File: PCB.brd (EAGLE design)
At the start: 127 x 44.5 mm, 45 parts, among them IC1 PIC16F1826/27SO, IC2 MAX3467CPA, U1 +12v, Y1 ASL-16.000MHZ-L-C-S-50-T

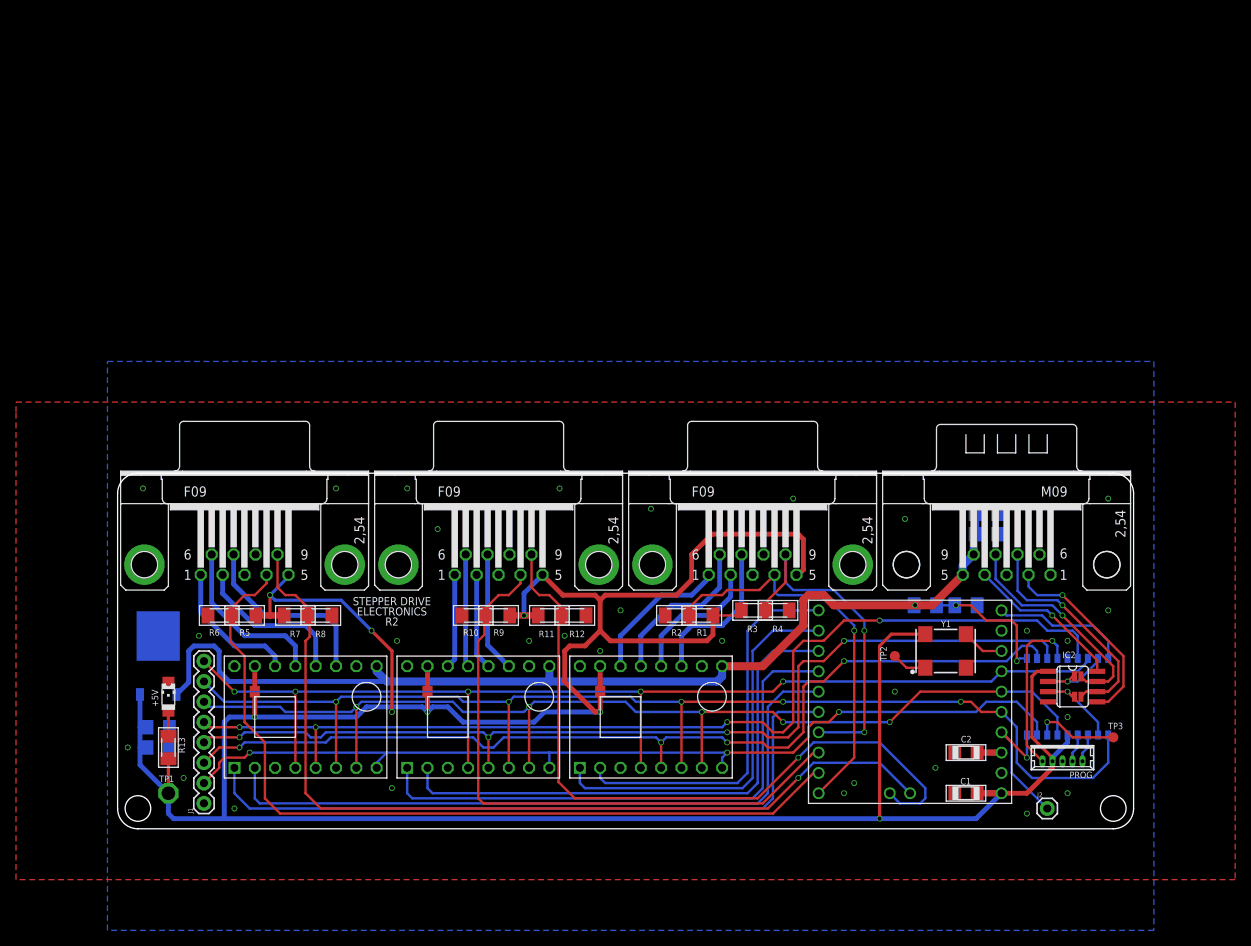
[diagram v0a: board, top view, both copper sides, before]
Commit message: Updating PCB design
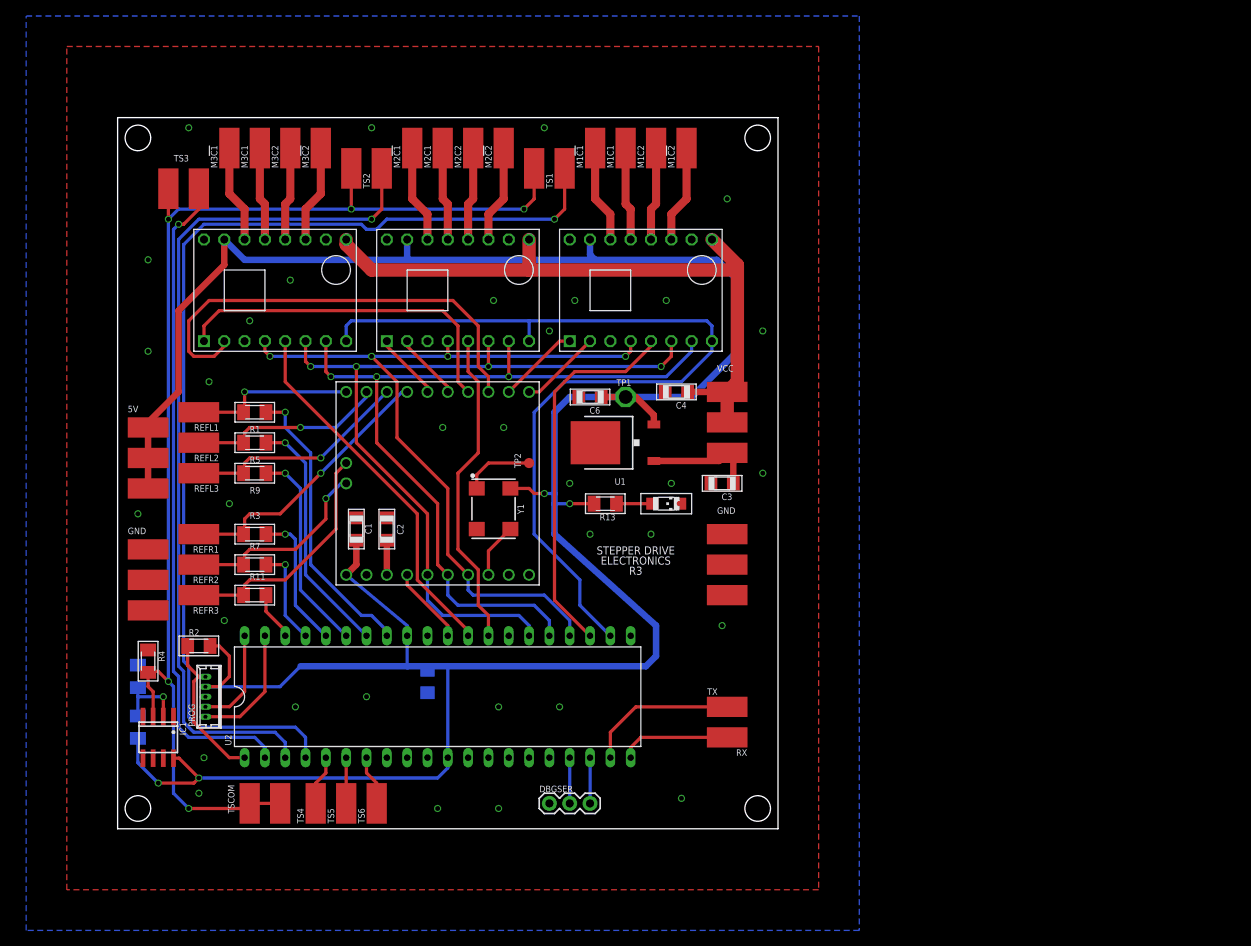
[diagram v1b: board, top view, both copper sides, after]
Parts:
- removed IC2: MAX3467CPA, maxim:SO08
- removed J1: (no value), SparkFun-Connectors:1X08
- removed J2: (no value), SparkFun-Connectors:1X01
- removed JP1, JP2, JP3, JP4, JP5: JUMPER-SMT_2_NO_NO-SILK, SparkFun-Jumpers:SMT-JUMPER_2_NO_NO-SILK
- removed R10, R12, R14, R15: (no value), resistor:M1206
- removed TP3: PTR1B1,27, testpad:B1,27
- removed X1, X2, X3: (no value), con-subd:F09HP
- removed X4: (no value), con-subd:M09H
- added 5V@1, 5V@2, 5V@3, GND@1, GND@2, GND@3, GND@4, GND@5, GND@6, M1!C1, M1!C2, M1C1, M1C2, M2!C1, M2!C2, M2C1, M2C2, M3!C1, M3!C2, M3C1, M3C2, REFL1, REFL2, REFL3, REFR1, REFR2, REFR3, RX, TS1, TS2, TS3, TS4, TS5, TS6, TSCOM@1, TSCOM@2, TSCOM@3, TSCOM@4, TSCOM@5, TX, VCC@1, VCC@2, VCC@3: WIREPADSMD2,54-5,08, wirepad:SMD2,54-5,08
- added DBGSER: (no value), SparkFun-Connectors:1X03
- added U2: PIC18F47Q84, FRC696:DIL40
- C3, C5: value (none) -> 0.1uF
- C4, C6: value (none) -> 1uF
- IC1: value PIC16F1826/27SO -> LM393D; device microchip:SO-18W -> linear:SO08
- PROG: value 53047-05 -> PIC-PROG047; device con-molex:53047-05 -> FRC696:53047-05
- R1, R11, R2, R3, R5, R7, R9: value (none) -> 5k
- R13: value (none) -> 330
- R4, R6: value (none) -> 10k
- R8: value (none) -> 2.2k
- moved IC1 113.8 mm to (5.08, 11.4), flipped to the top
- moved PROG 107.0 mm to (11.4, 16.5), turned to 90 degrees
- moved C1 83.0 mm to (29.8, 37.5), turned to 90 degrees
- moved R4 79.0 mm to (3.81, 21.0), turned to 270 degrees
- moved C2 77.6 mm to (33.7, 37.5), turned to 270 degrees
- moved TP1 75.6 mm to (63.5, 54.0)
- moved C6 69.5 mm to (59.1, 54.0), flipped to the top
- moved U$1 66.8 mm to (38.7, 43.2), turned to 90 degrees
- moved LED1 66.7 mm to (68.6, 40.6), turned to 270 degrees
- moved U1 63.1 mm to (62.2, 48.3), flipped to the top, turned to 90 degrees
- moved R3 63.0 mm to (17.1, 36.8), turned to 0 degrees
- moved R13 62.5 mm to (61.0, 40.6), turned to 180 degrees
- moved R1 61.4 mm to (17.1, 52.1)
- moved R2 59.8 mm to (10.2, 22.9)
- moved Y1 59.2 mm to (47.0, 40.0), turned to 270 degrees
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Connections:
- removed net N$25: IC1.16, TP3.TP
- removed net N$29: DRV2.P$15, JP4.1
- removed net N$30: DRV1.P$15, JP3.1
- removed net N$31: DRV3.P$15, JP5.1
- removed net N$33: IC1.1, R14.1, R15.2
- removed net RXN: IC2.7, JP2.1, X4.8
- removed net RXP: IC2.8, X4.4
- removed net TXN: IC2.6, JP1.1, X4.7
- removed net TXP: IC2.5, X4.2
- new net DBGRX: DBGSER.3, U2.18
- new net DBGTX: DBGSER.2, U2.17
- new net N$26: IC1.2, R6.1, R8.2
- new net REFL1P: R1.2, U2.33
- new net REFL2P: R5.2, U2.34
- new net REFL3P: R9.2, U2.35
- new net REFR1P: R3.2, U2.36
- new net REFR2P: R7.2, U2.37
- new net REFR3P: R11.2, U2.38
- new net TS1: TS1.1, U2.4
- new net TS2: TS2.1, U2.3
- new net TS3: TS3.1, U2.2
- new net TS4: TS4.1, U2.5
- new net TS5: TS5.1, U2.6
- new net TS6: TS6.1, U2.7
- new net TSCOM: IC1.3, R4.2, TSCOM@1.1, TSCOM@2.1, TSCOM@3.1, TSCOM@4.1, TSCOM@5.1
- new net TSOUT: IC1.1
- net +5V: now also 5V@1.1, 5V@2.1, 5V@3.1, DRV1.P$15, DRV2.P$15, DRV3.P$15, IC1.8, R2.2, R6.2, U2.11, U2.32; no longer IC1.14, IC2.1, JP3.2, JP4.2, JP5.2, R1.2, R11.2, R3.2, R5.2, R7.2, R9.2, X1.5, X2.5, X3.5
- net D1CS: now also U2.23; no longer IC1.2, J1.3
- net D2CS: now also U2.28; no longer IC1.6, J1.5
- net D3CS: now also U2.29; no longer IC1.3, J1.4
- net DRVEN: now also U2.22; no longer IC1.17, J1.2
- net GND: now also DBGSER.1, GND@1.1, GND@2.1, GND@3.1, GND@4.1, GND@5.1, GND@6.1, IC1.4, IC1.6, U2.12, U2.31; no longer IC2.4, J1.1, R10.1, R12.1, R15.1, R2.1, R6.1, X1.8, X2.8, X3.8, X4.1, X4.6
- net MCCS: now also U2.30; no longer IC1.18, J2.1
- net MCINT: no longer IC1.9
- net MISO: now also U2.24; no longer IC1.7, J1.8
- net MOSI: now also U2.25; no longer IC1.15, J1.6
- net N$10: now also M1!C1.1; no longer X1.1
- net N$11: now also M1!C2.1; no longer X1.7
- net N$12: now also M2!C1.1; no longer X2.1
- net N$13: now also M2C2.1; no longer X2.2
- net N$14: now also M2!C2.1; no longer X2.7
- net N$15: now also M2C1.1; no longer X2.6
- net N$16: now also M3!C1.1; no longer X3.1
- net N$17: now also M3C2.1; no longer X3.2
- net N$18: now also M3C1.1; no longer X3.6
- net N$19: now also M3!C2.1; no longer X3.7
- net N$20: now also PROG.4, U2.40; no longer IC1.4, PROG.1
- net N$21: now also PROG.1, R2.1, U2.1; no longer IC1.13, PROG.4
- net N$22: now also U2.39; no longer IC1.12
- net N$8: now also M1C1.1; no longer X1.6
- net N$9: now also M1C2.1; no longer X1.2
- net REFL1: now also REFL1.1; no longer R2.2, X1.4
- net REFL2: now also REFL2.1; no longer R6.2, X2.4
- net REFL3: now also REFL3.1; no longer R10.2, X3.4
- net REFR1: now also REFR1.1; no longer R4.2, X1.9
- net REFR2: now also REFR2.1; no longer R8.2, X2.9
- net REFR3: now also REFR3.1; no longer R12.2, X3.9
- net SCK: now also U2.26; no longer IC1.10, J1.7
- net UARTRX: now also RX.1, U2.20; no longer IC1.8, IC2.2, JP2.2
- net UARTTX: now also TX.1, U2.19; no longer IC1.11, IC2.3, JP1.2
- net VCC: now also VCC@1.1, VCC@2.1, VCC@3.1; no longer R14.2, X4.5, X4.9
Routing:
- net TSCOM: track 0.00 -> 154.8 mm, vias 0 -> 5
- net TS1: track 0.00 -> 132.6 mm, vias 0 -> 1
- net TS2: track 0.00 -> 108.3 mm, vias 0 -> 1
- net D2CS: track 130.0 -> 40.0 mm, vias 4 -> 0
- net REFR2: track 113.0 -> 24.8 mm
- net TS3: track 0.00 -> 82.4 mm, vias 0 -> 1
- net REFL2: track 104.7 -> 24.6 mm, vias 0 -> 1
- net N$4: track 87.9 -> 8.45 mm
- net N$3: track 86.7 -> 8.45 mm
- net D3CS: track 122.3 -> 46.3 mm, vias 4 -> 0
- net D1CS: track 120.5 -> 47.4 mm, vias 4 -> 0
- net REFR3: track 89.8 -> 30.0 mm, vias 1 -> 0
- net REFL3: track 76.5 -> 28.4 mm, vias 0 -> 1
- net SCK: track 150.7 -> 104.2 mm, vias 5 -> 4
- net MISO: track 142.6 -> 101.1 mm, vias 5 -> 4
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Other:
- board size 127 x 44.5 mm -> 82.5 x 88.9 mm
- board text added: "5V"
- board text added: "GND"
- board text added: "R3"
- board text added: "TSCOM"
- board text added: "VCC"
- board text removed: "+5V"
- board text removed: "R2"
